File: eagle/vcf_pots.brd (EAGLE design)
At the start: 100 x 80 mm, 18 parts, among them P1 P0915N, P10 P0915N, P2 P0915N, P3 P0915N, P4 P0915N, P5 P0915N, P6 P0915N, P7 P0915N, P8 P0915N, P9 P0915N, X2 87758-0216, X3 87758-0216

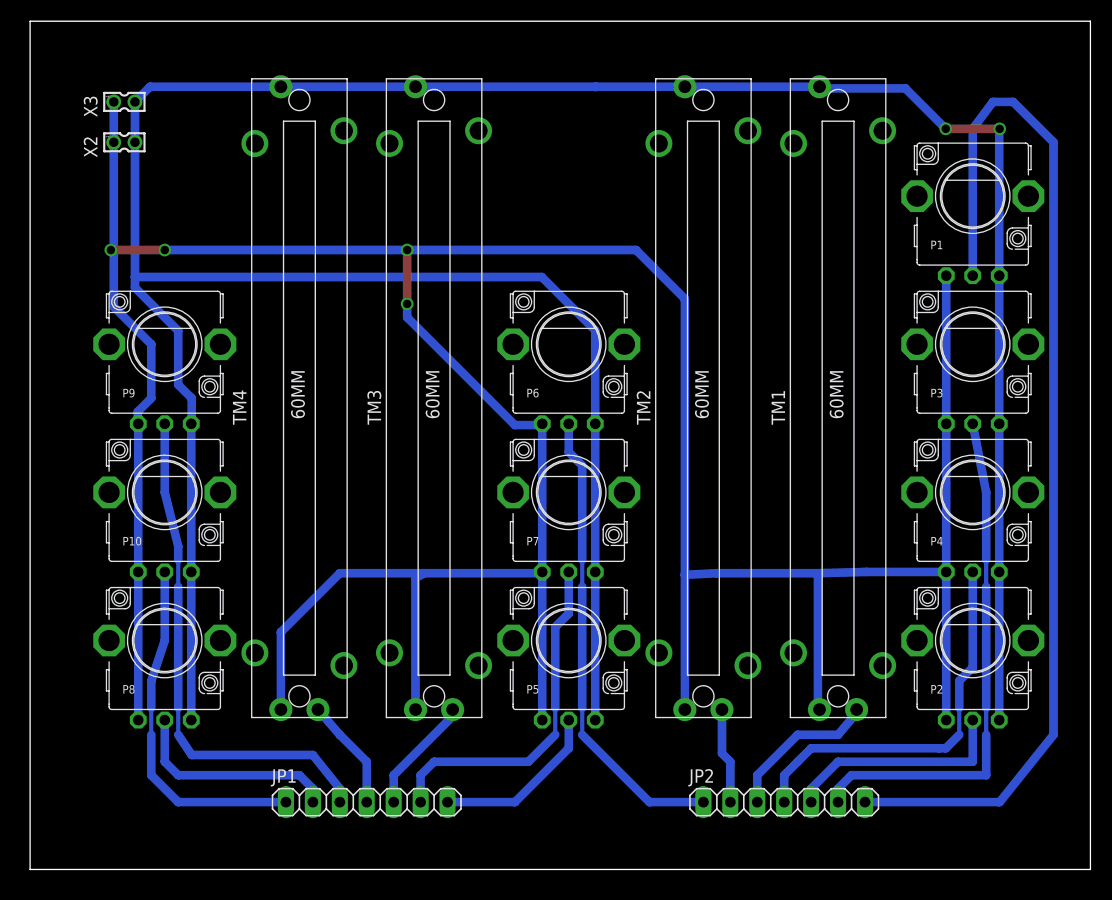
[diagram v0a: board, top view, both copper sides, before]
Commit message: vcf pot board
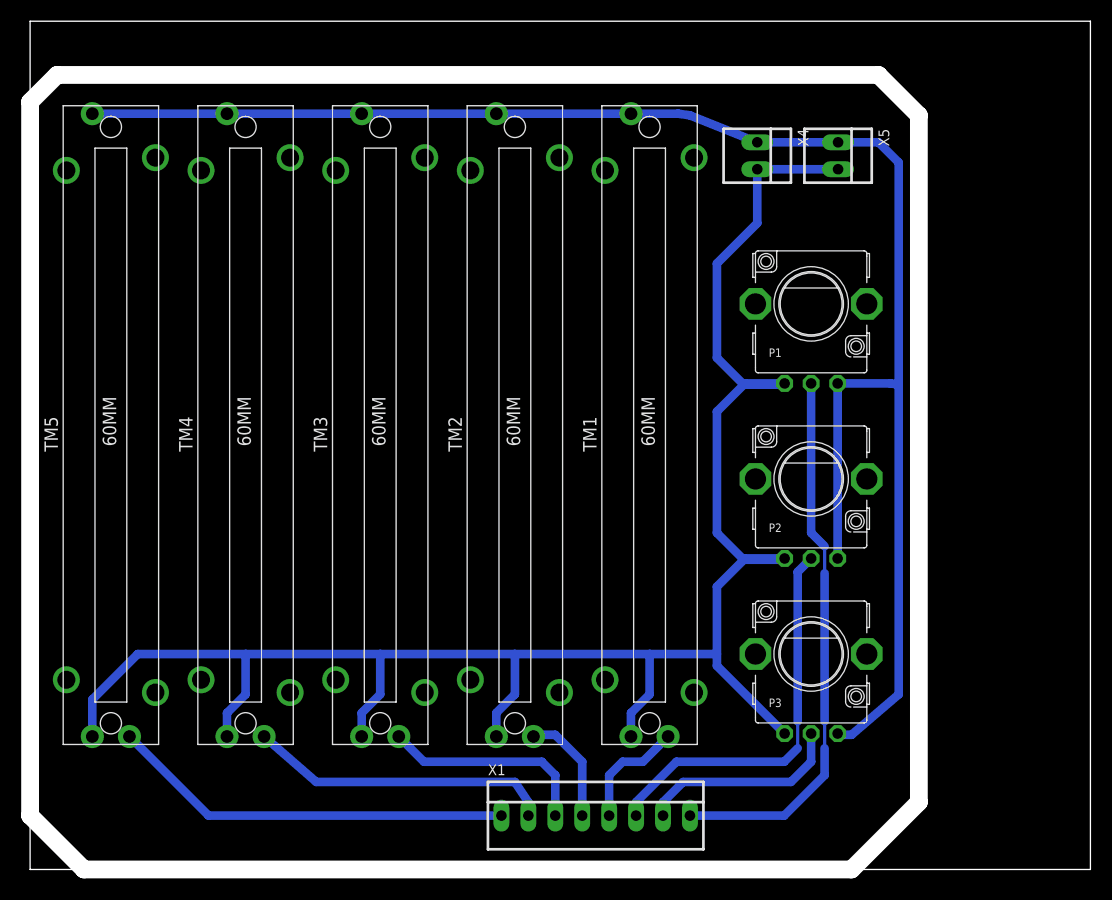
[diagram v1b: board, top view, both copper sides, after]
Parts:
- removed JP1, JP2: (no value), pinhead:1X07
- removed P10, P4, P5, P6, P7, P8, P9: P0915N, pot-tt_electronics:P0915N
- removed X2, X3: 87758-0216, con-molex:87758-0216
- added TM5: (no value), stefan-lochbrunner_EAGLE_master_custom%20libraries_potentiometers_Bourns%20PTA%20series_Bourns%20PTA%20series:SLIDEPOT-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
- added X1: 22-23-2081, con-molex:22-23-2081
- added X4, X5: 22-23-2021, con-molex:22-23-2021
- moved P3 32.9 mm to (73.7, 20.3)
- moved P2 21.6 mm to (73.7, 36.8)
- moved P1 18.3 mm to (73.7, 53.3)
- moved TM1 18.0 mm to (58.4, 41.9)
- moved TM2 18.0 mm to (45.7, 41.9)
- moved TM3 5.68 mm to (33.0, 41.9)
- moved TM4 5.68 mm to (20.3, 41.9)
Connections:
- removed net N$10: JP2.4, P4.S
- removed net N$11: JP1.4, TM4.WIPER
- removed net N$12: JP1.5, TM3.WIPER
- removed net N$13: JP2.2, TM2.WIPER
- removed net N$14: JP2.3, TM1.WIPER
- removed net N$9: JP2.7, P1.S
- net +5V: now also TM5.B, X4.1, X5.1; no longer P10.E, P4.E, P5.E, P6.E, P7.E, P8.E, P9.E, X2.2, X3.2
- net GND: now also TM5.A, X4.2, X5.2; no longer P10.A, P4.A, P5.A, P6.A, P7.A, P8.A, P9.A, X2.1, X3.1
- net N$1: now also P1.S, X1.8; no longer JP1.1, P10.S
- net N$2: now also P2.S, X1.6; no longer JP2.1, P6.S
- net N$3: now also P3.S, X1.7; no longer JP2.5, P2.S
- net N$4: now also TM1.WIPER, X1.5; no longer JP1.6, P7.S
- net N$5: now also TM2.WIPER, X1.4; no longer JP2.6, P3.S
- net N$6: now also TM3.WIPER, X1.3; no longer JP1.2, P8.S
- net N$7: now also TM4.WIPER, X1.2; no longer JP1.3, P9.S
- net N$8: now also TM5.WIPER, X1.1; no longer JP1.7, P5.S
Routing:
- net GND: track 334.4 -> 183.1 mm, vias 4 -> 0
- net +5V: track 282.4 -> 158.1 mm, vias 2 -> 0
- net N$9: track 101.0 -> 0.00 mm
- net N$5: track 49.0 -> 10.8 mm
- net N$10: track 36.5 -> 0.00 mm
- net N$8: track 16.2 -> 38.2 mm
- net N$4: track 32.7 -> 10.9 mm
- net N$7: track 48.5 -> 28.8 mm
- net N$1: track 33.1 -> 51.8 mm
- net N$14: track 14.8 -> 0.00 mm
- net N$12: track 11.0 -> 0.00 mm
- net N$11: track 10.5 -> 0.00 mm
- net N$13: track 9.06 -> 0.00 mm
- net N$2: track 43.9 -> 37.0 mm
- net N$3: track 21.5 -> 19.5 mm
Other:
- outline, holes or cut-outs redrawn
